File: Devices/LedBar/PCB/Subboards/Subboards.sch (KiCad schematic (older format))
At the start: 3 parts

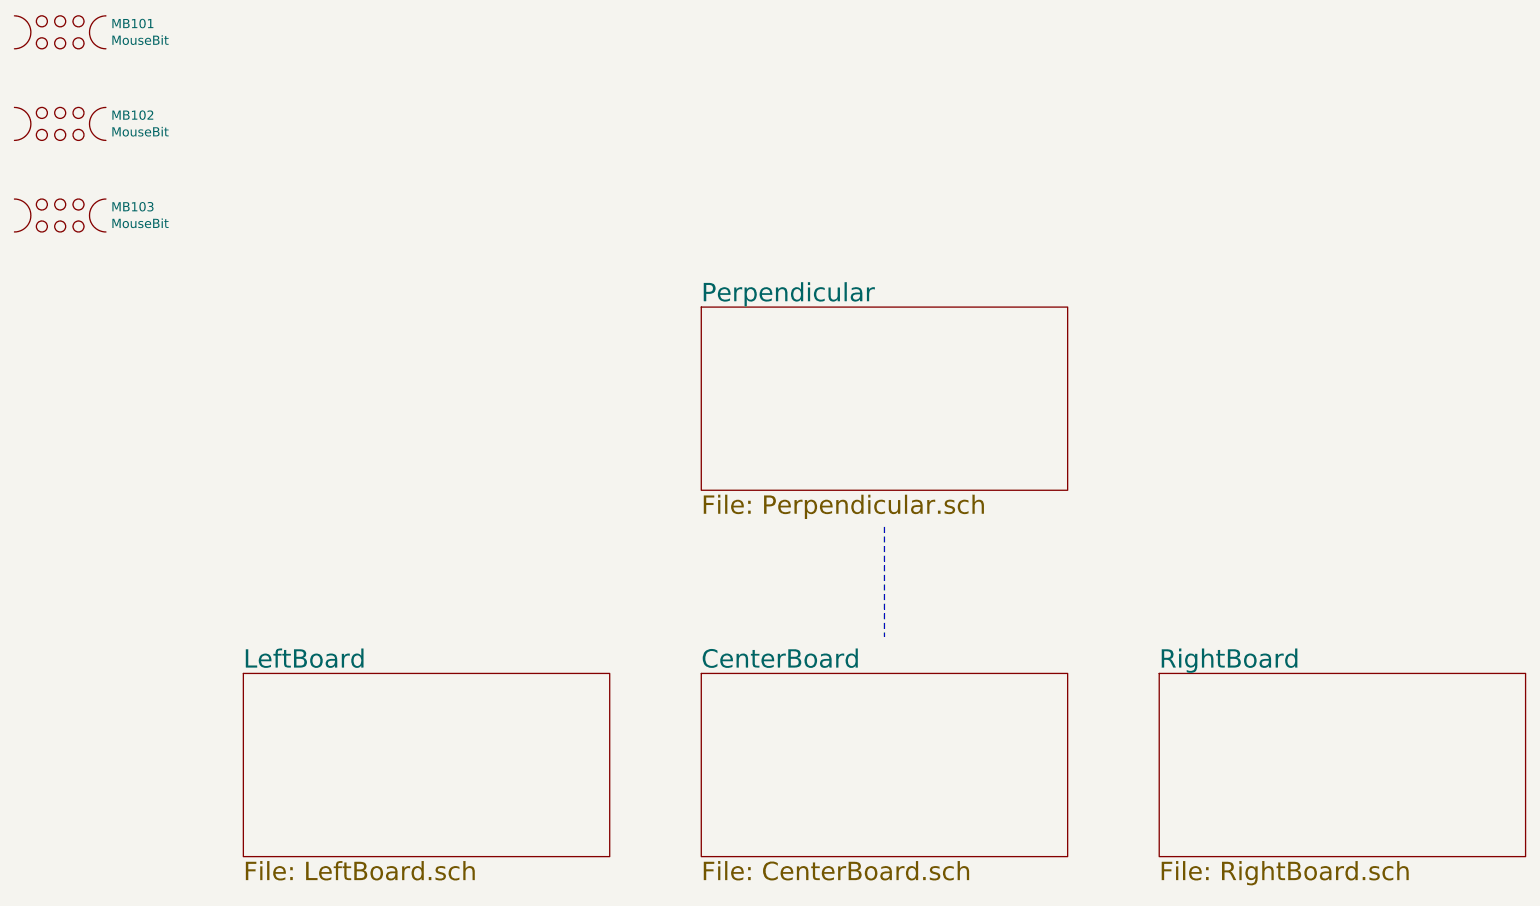
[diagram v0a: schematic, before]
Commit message: Releasing RGBW-LEDBar v2.0
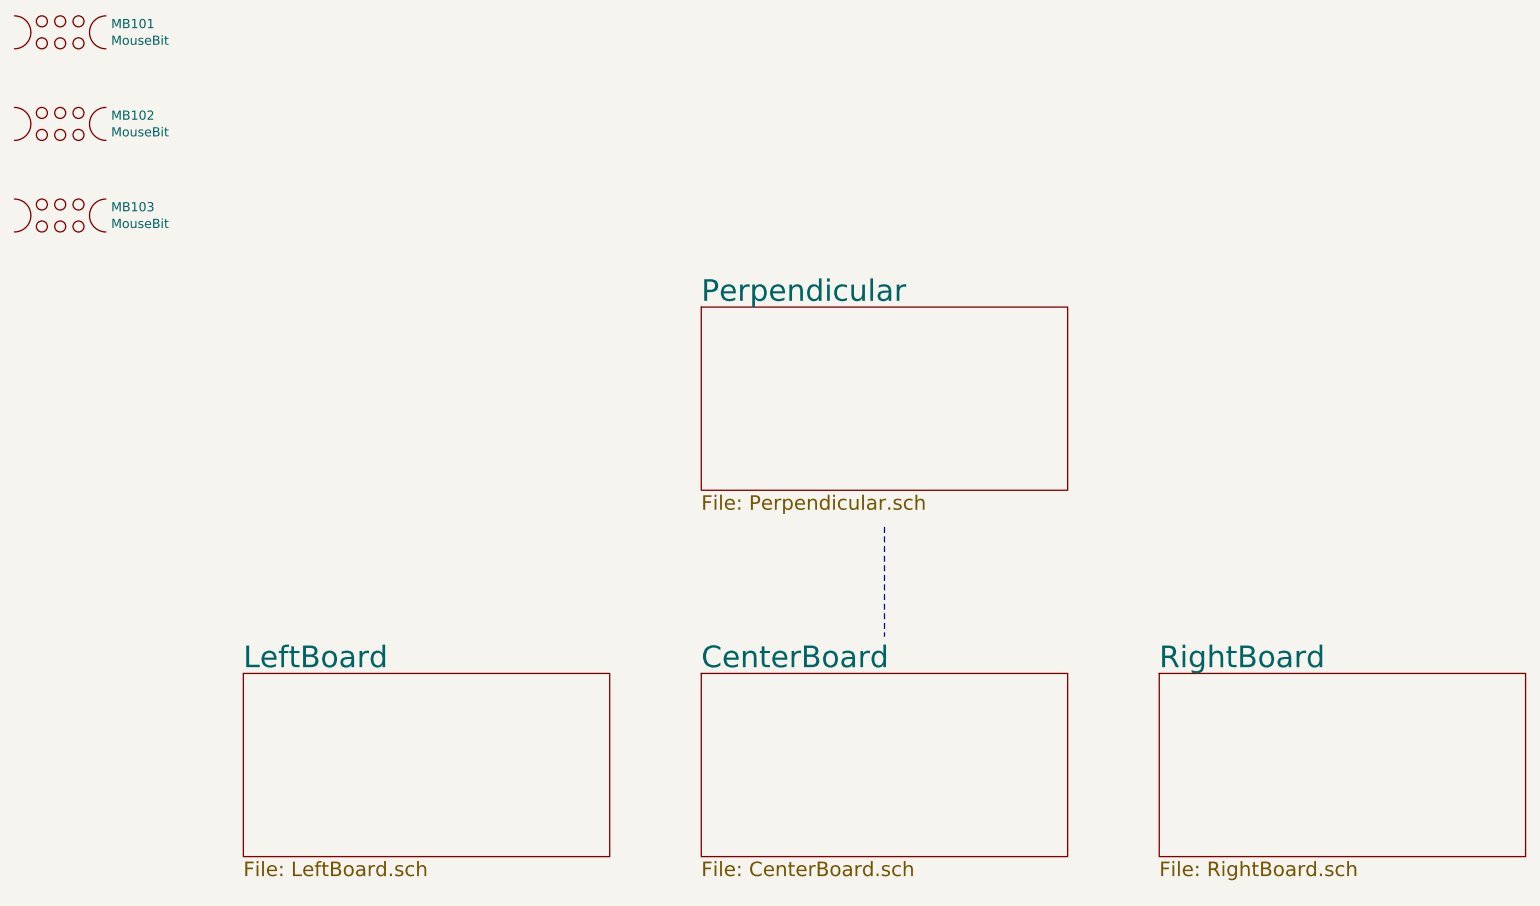
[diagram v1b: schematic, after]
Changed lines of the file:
@@
 encoding utf-8
 Sheet 1 5
-Title ""
-Date ""
-Rev ""
-Comp ""
-Comment1 ""
+Title "LedBar - MainBoard"
+Date "2022-12-06"
+Rev "2.0"
+Comp "Roel Drost"
+Comment1 "GNU General Public License v3.0"
 Comment2 ""
 Comment3 ""
-Comment4 ""
+Comment4 "4 channel RGBW LED bar, Arduino compatible with isolated half duplex RS485."
 $EndDescr
 $Sheet
 S 5000 5000 2000 1000
 U 6371587E
-F0 "CenterBoard" 100
-F1 "CenterBoard.sch" 100
+F0 "CenterBoard" 118
+F1 "CenterBoard.sch" 79
 $EndSheet
 $Sheet
 S 7500 5000 2000 1000
 U 637158E2
-F0 "RightBoard" 100
-F1 "RightBoard.sch" 100
+F0 "RightBoard" 118
+F1 "RightBoard.sch" 79
 $EndSheet
 $Sheet
 S 2500 5000 2000 1000
 U 6371595F
-F0 "LeftBoard" 100
-F1 "LeftBoard.sch" 100
+F0 "LeftBoard" 118
+F1 "LeftBoard.sch" 79
 $EndSheet
 $Sheet
 S 5000 3000 2000 1000
 U 637159B2
-F0 "Perpendicular" 100
-F1 "Perpendicular.sch" 100
+F0 "Perpendicular" 118
+F1 "Perpendicular.sch" 79
 $EndSheet
 Wire Notes Line
